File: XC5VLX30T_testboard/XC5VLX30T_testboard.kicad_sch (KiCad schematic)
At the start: 19 parts, among them J1 Conn_01x35_Pin, J2 Conn_01x35_Pin, J3 Conn_01x35_Pin, J4 Conn_01x35_Pin, J5 Conn_01x35_Pin, J6 Conn_01x35_Pin, J7 Conn_01x35_Pin, J8 Conn_01x35_Pin, U1 XC5VLX30T-1FFG665C, X1 SG-5032CCN

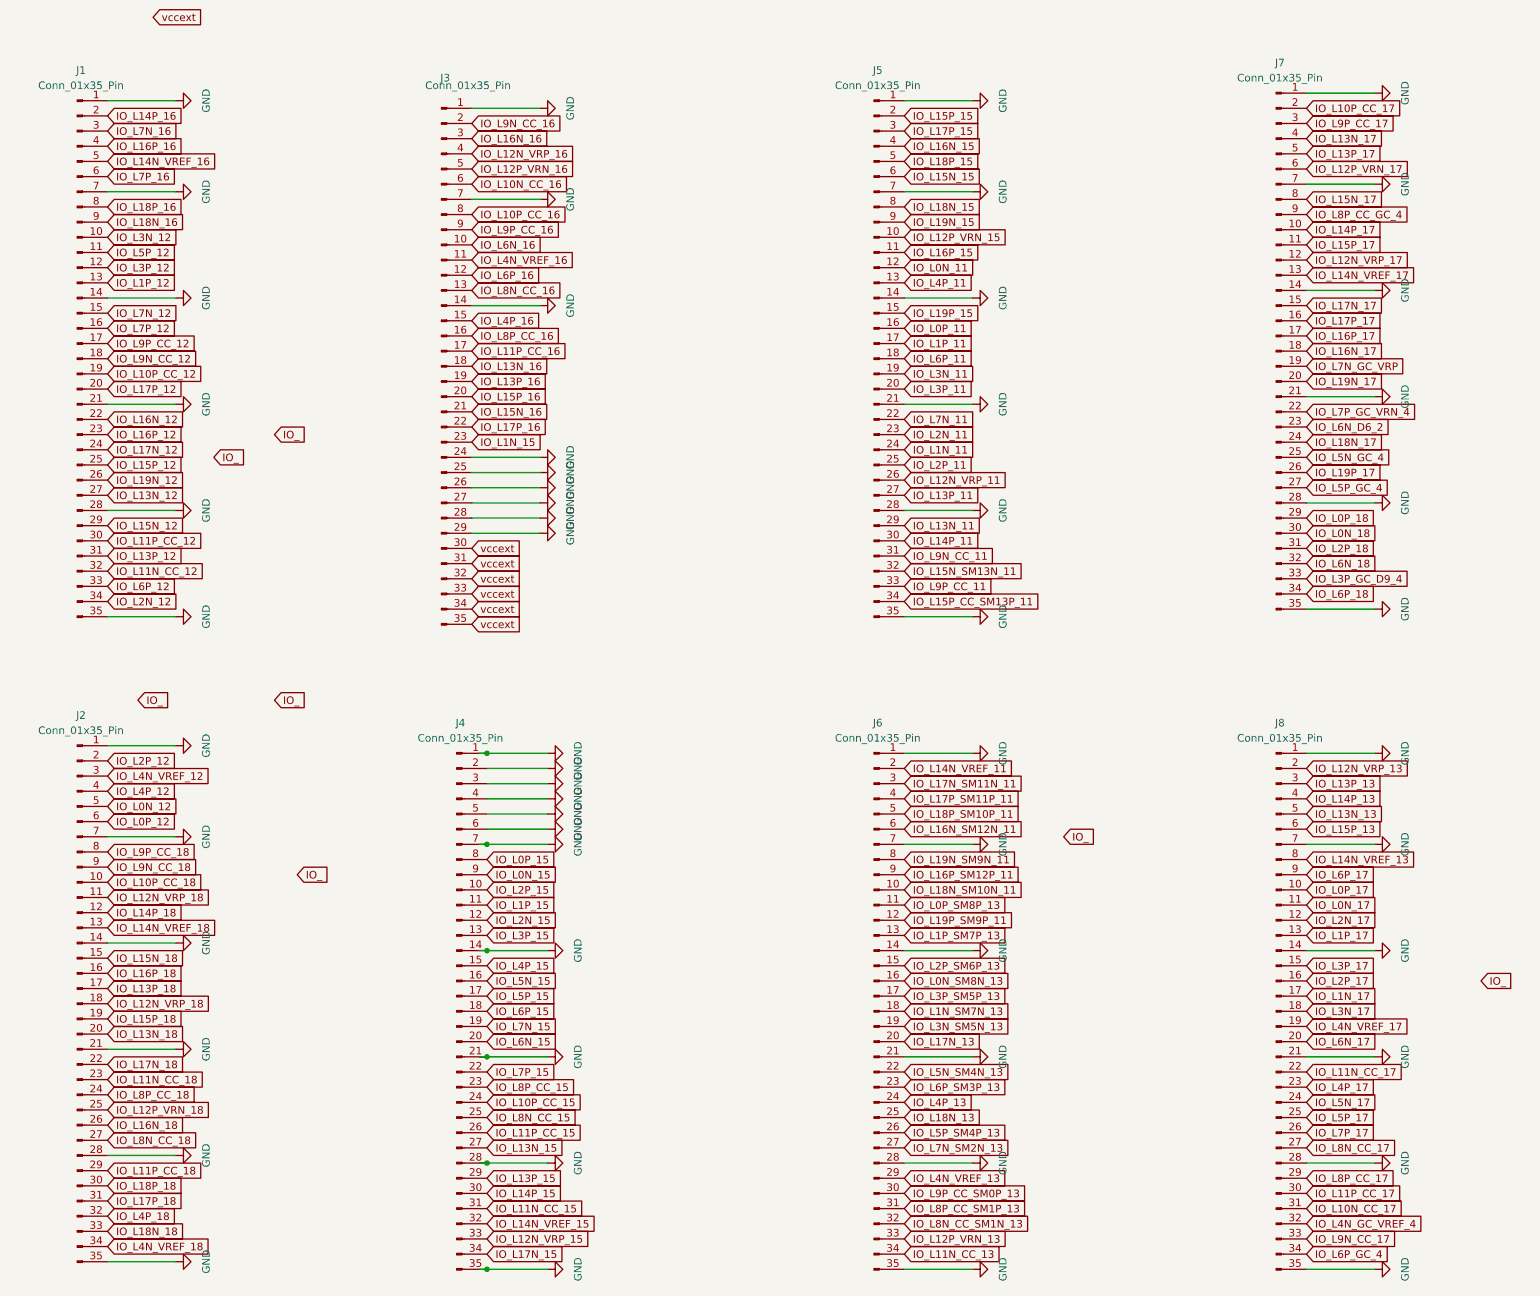
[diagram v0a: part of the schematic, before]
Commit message: more routing
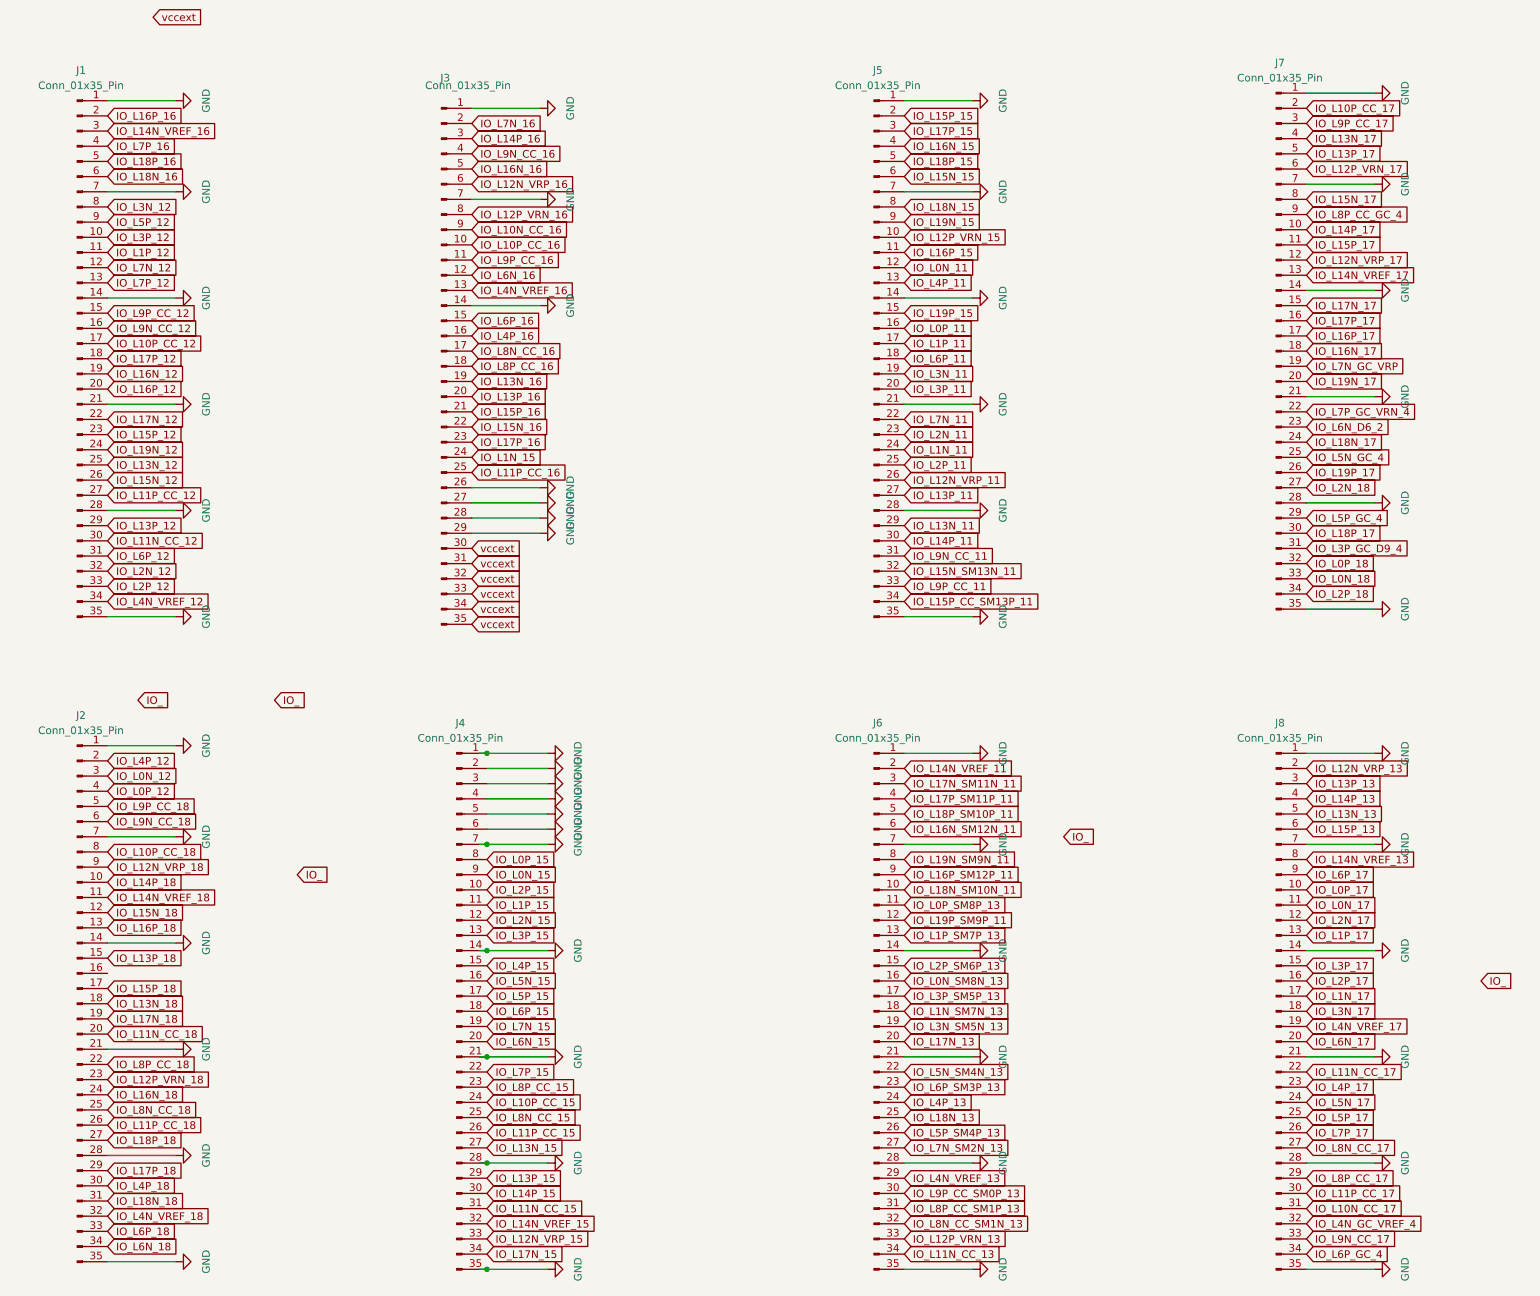
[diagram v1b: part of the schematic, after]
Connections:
- net GND: no longer J3.24 (Pin_24), J3.25 (Pin_25)
- net IO_L0N_12: now also J2.3 (Pin_3); no longer J2.5 (Pin_5)
- net IO_L0N_18: now also J7.33 (Pin_33); no longer J7.30 (Pin_30)
- net IO_L0P_12: now also J2.4 (Pin_4); no longer J2.6 (Pin_6)
- net IO_L0P_18: now also J7.32 (Pin_32); no longer J7.29 (Pin_29)
- net IO_L10N_CC_16: now also J3.9 (Pin_9); no longer J3.6 (Pin_6)
- net IO_L10P_CC_12: now also J1.17 (Pin_17); no longer J1.19 (Pin_19)
- net IO_L10P_CC_16: now also J3.10 (Pin_10); no longer J3.8 (Pin_8)
- net IO_L10P_CC_18: now also J2.8 (Pin_8); no longer J2.10 (Pin_10)
- net IO_L11N_CC_12: now also J1.30 (Pin_30); no longer J1.32 (Pin_32)
- net IO_L11N_CC_18: now also J2.20 (Pin_20); no longer J2.23 (Pin_23)
- net IO_L11P_CC_12: now also J1.27 (Pin_27); no longer J1.30 (Pin_30)
- net IO_L11P_CC_16: now also J3.25 (Pin_25); no longer J3.17 (Pin_17)
- net IO_L11P_CC_18: now also J2.26 (Pin_26); no longer J2.29 (Pin_29)
- net IO_L12N_VRP_16: now also J3.6 (Pin_6); no longer J3.4 (Pin_4)
- net IO_L12N_VRP_18: now also J2.9 (Pin_9); no longer J2.11 (Pin_11), J2.18 (Pin_18)
- net IO_L12P_VRN_16: now also J3.8 (Pin_8); no longer J3.5 (Pin_5)
- net IO_L12P_VRN_18: now also J2.23 (Pin_23); no longer J2.25 (Pin_25)
- net IO_L13N_12: now also J1.25 (Pin_25); no longer J1.27 (Pin_27)
- net IO_L13N_16: now also J3.19 (Pin_19); no longer J3.18 (Pin_18)
- net IO_L13N_18: now also J2.18 (Pin_18); no longer J2.20 (Pin_20)
- net IO_L13P_12: now also J1.29 (Pin_29); no longer J1.31 (Pin_31)
- net IO_L13P_16: now also J3.20 (Pin_20); no longer J3.19 (Pin_19)
- net IO_L13P_18: now also J2.15 (Pin_15); no longer J2.17 (Pin_17)
- net IO_L14N_VREF_16: now also J1.3 (Pin_3); no longer J1.5 (Pin_5)
- net IO_L14N_VREF_18: now also J2.11 (Pin_11); no longer J2.13 (Pin_13)
- net IO_L14P_16: now also J3.3 (Pin_3); no longer J1.2 (Pin_2)
- net IO_L14P_18: now also J2.10 (Pin_10); no longer J2.12 (Pin_12)
- net IO_L15N_12: now also J1.26 (Pin_26); no longer J1.29 (Pin_29)
- net IO_L15N_16: now also J3.22 (Pin_22); no longer J3.21 (Pin_21)
- net IO_L15N_18: now also J2.12 (Pin_12); no longer J2.15 (Pin_15)
- net IO_L15P_12: now also J1.23 (Pin_23); no longer J1.25 (Pin_25)
- net IO_L15P_16: now also J3.21 (Pin_21); no longer J3.20 (Pin_20)
- net IO_L15P_18: now also J2.17 (Pin_17); no longer J2.19 (Pin_19)
- net IO_L16N_12: now also J1.19 (Pin_19); no longer J1.22 (Pin_22)
- net IO_L16N_16: now also J3.5 (Pin_5); no longer J3.3 (Pin_3)
- net IO_L16N_18: now also J2.24 (Pin_24); no longer J2.26 (Pin_26)
- net IO_L16P_12: now also J1.20 (Pin_20); no longer J1.23 (Pin_23)
- net IO_L16P_16: now also J1.2 (Pin_2); no longer J1.4 (Pin_4)
- net IO_L16P_18: now also J2.13 (Pin_13); no longer J2.16 (Pin_16)
- net IO_L17N_12: now also J1.22 (Pin_22); no longer J1.24 (Pin_24)
- net IO_L17N_18: now also J2.19 (Pin_19); no longer J2.22 (Pin_22)
- net IO_L17P_12: now also J1.18 (Pin_18); no longer J1.20 (Pin_20)
- net IO_L17P_16: now also J3.23 (Pin_23); no longer J3.22 (Pin_22)
- net IO_L17P_18: now also J2.29 (Pin_29); no longer J2.31 (Pin_31)
- net IO_L18N_16: now also J1.6 (Pin_6); no longer J1.9 (Pin_9)
- net IO_L18N_18: now also J2.31 (Pin_31); no longer J2.33 (Pin_33)
- net IO_L18P_16: now also J1.5 (Pin_5); no longer J1.8 (Pin_8)
- net IO_L18P_17: now also J7.30 (Pin_30)
- net IO_L18P_18: now also J2.27 (Pin_27); no longer J2.30 (Pin_30)
- net IO_L19N_12: now also J1.24 (Pin_24); no longer J1.26 (Pin_26)
- net IO_L1N_15: now also J3.24 (Pin_24); no longer J3.23 (Pin_23)
- net IO_L1P_12: now also J1.11 (Pin_11); no longer J1.13 (Pin_13)
- net IO_L2N_12: now also J1.32 (Pin_32); no longer J1.34 (Pin_34)
- net IO_L2N_18: now also J7.27 (Pin_27)
- net IO_L2P_12: now also J1.33 (Pin_33); no longer J2.2 (Pin_2)
- net IO_L2P_18: now also J7.34 (Pin_34); no longer J7.31 (Pin_31)
- net IO_L3N_12: now also J1.8 (Pin_8); no longer J1.10 (Pin_10)
- net IO_L3P_12: now also J1.10 (Pin_10); no longer J1.12 (Pin_12)
- net IO_L3P_GC_D9_4: now also J7.31 (Pin_31); no longer J7.33 (Pin_33)
- net IO_L4N_VREF_12: now also J1.34 (Pin_34); no longer J2.3 (Pin_3)
- net IO_L4N_VREF_16: now also J3.13 (Pin_13); no longer J3.11 (Pin_11)
- net IO_L4N_VREF_18: now also J2.32 (Pin_32); no longer J2.34 (Pin_34)
- net IO_L4P_12: now also J2.2 (Pin_2); no longer J2.4 (Pin_4)
- net IO_L4P_16: now also J3.16 (Pin_16); no longer J3.15 (Pin_15)
- net IO_L4P_18: now also J2.30 (Pin_30); no longer J2.32 (Pin_32)
- net IO_L5P_12: now also J1.9 (Pin_9); no longer J1.11 (Pin_11)
- net IO_L5P_GC_4: now also J7.29 (Pin_29); no longer J7.27 (Pin_27)
- net IO_L6N_16: now also J3.12 (Pin_12); no longer J3.10 (Pin_10)
- net IO_L6N_18: now also J2.34 (Pin_34); no longer J7.32 (Pin_32)
- net IO_L6P_12: now also J1.31 (Pin_31); no longer J1.33 (Pin_33)
- net IO_L6P_16: now also J3.15 (Pin_15); no longer J3.12 (Pin_12)
- net IO_L6P_18: now also J2.33 (Pin_33); no longer J7.34 (Pin_34)
- net IO_L7N_12: now also J1.12 (Pin_12); no longer J1.15 (Pin_15)
- net IO_L7N_16: now also J3.2 (Pin_2); no longer J1.3 (Pin_3)
- net IO_L7P_12: now also J1.13 (Pin_13); no longer J1.16 (Pin_16)
- net IO_L7P_16: now also J1.4 (Pin_4); no longer J1.6 (Pin_6)
- net IO_L8N_CC_16: now also J3.17 (Pin_17); no longer J3.13 (Pin_13)
- net IO_L8N_CC_18: now also J2.25 (Pin_25); no longer J2.27 (Pin_27)
- net IO_L8P_CC_16: now also J3.18 (Pin_18); no longer J3.16 (Pin_16)
- net IO_L8P_CC_18: now also J2.22 (Pin_22); no longer J2.24 (Pin_24)
- net IO_L9N_CC_12: now also J1.16 (Pin_16); no longer J1.18 (Pin_18)
- net IO_L9N_CC_16: now also J3.4 (Pin_4); no longer J3.2 (Pin_2)
- net IO_L9N_CC_18: now also J2.6 (Pin_6); no longer J2.9 (Pin_9)
- net IO_L9P_CC_12: now also J1.15 (Pin_15); no longer J1.17 (Pin_17)
- net IO_L9P_CC_16: now also J3.11 (Pin_11); no longer J3.9 (Pin_9)
- net IO_L9P_CC_18: now also J2.5 (Pin_5); no longer J2.8 (Pin_8)
